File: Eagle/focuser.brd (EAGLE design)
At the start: 193 x 147.3 mm, 72 parts, among them IC1 L293D, IC2 L293D, IC4 L293D, IC5 7809, IC6 ULN2003AN, J5 RJ11, K1 G5L, K2 G5L, K3 G5L, K4 G5L, K5 G5L, Q1 IRFN44Z, Q2 IRFN44Z, Q3 IRFN44Z, Q4 IRFN44Z, U1 ARDUINO-MEGAFULL, X1 STEPPER1, X2 STEPPER2, X3 TOBU3, X4 TOBU3, X5 TOBU3, X6 TOBU3

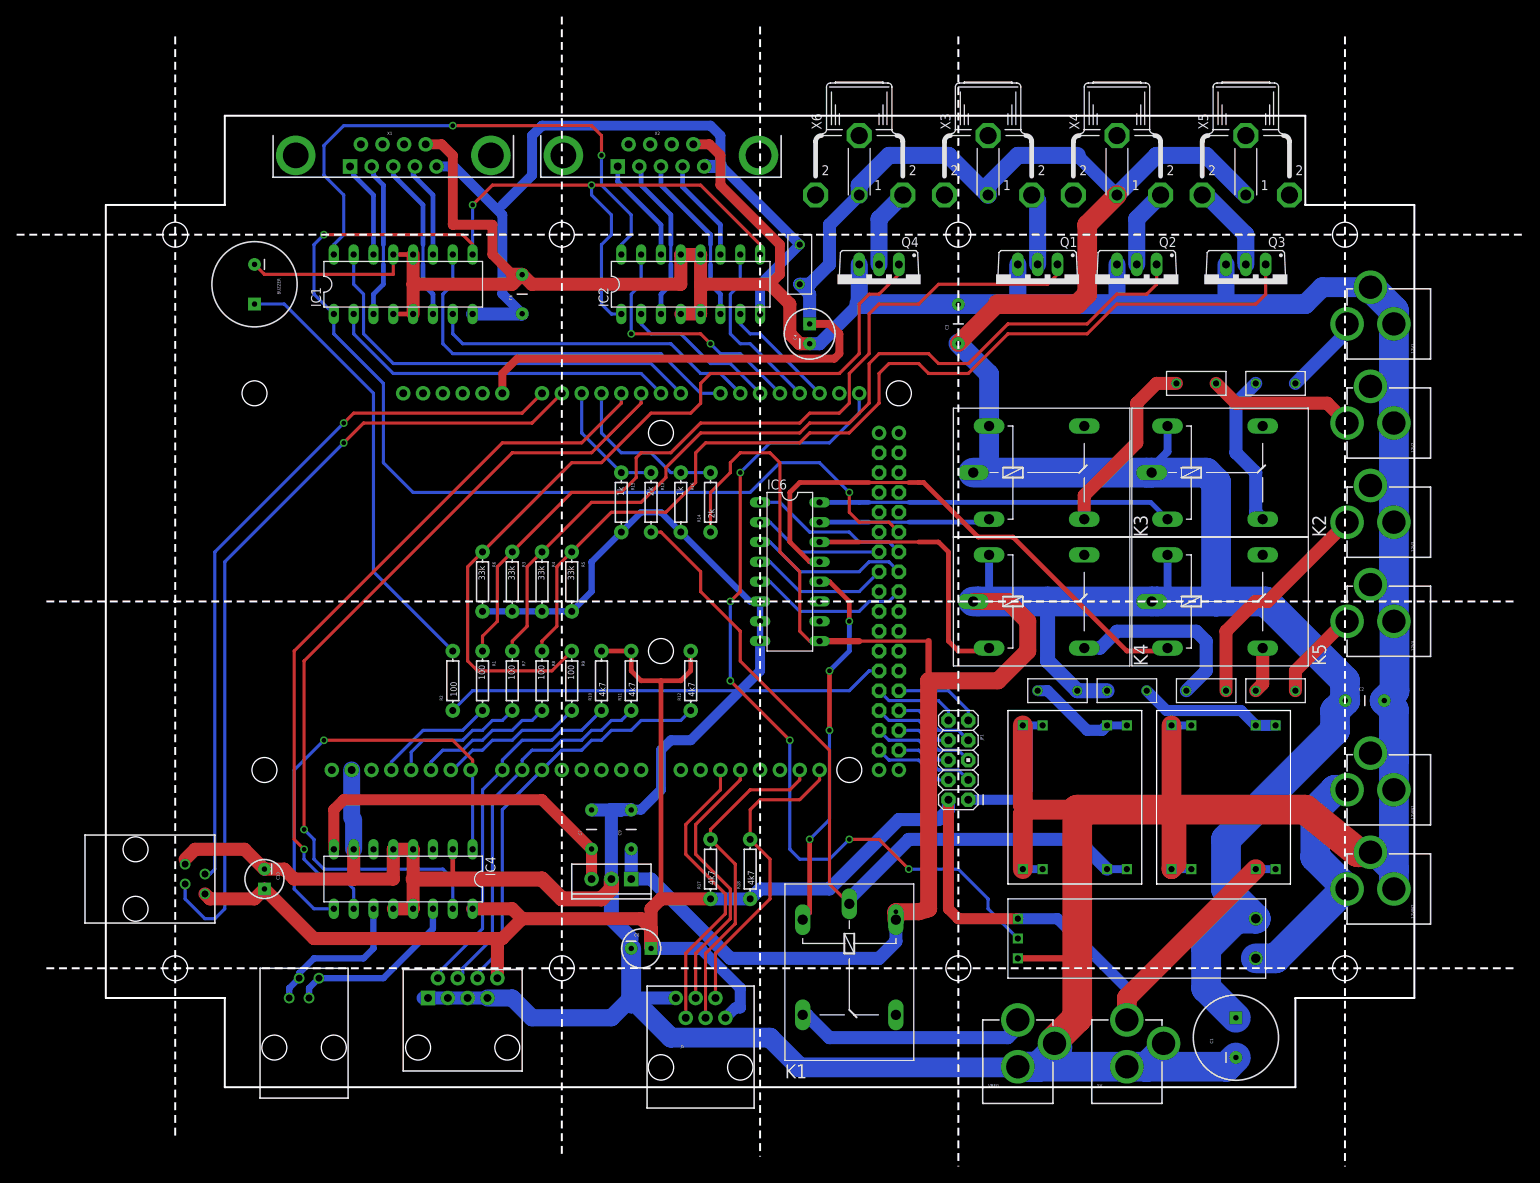
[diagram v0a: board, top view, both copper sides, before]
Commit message: PCB fixes
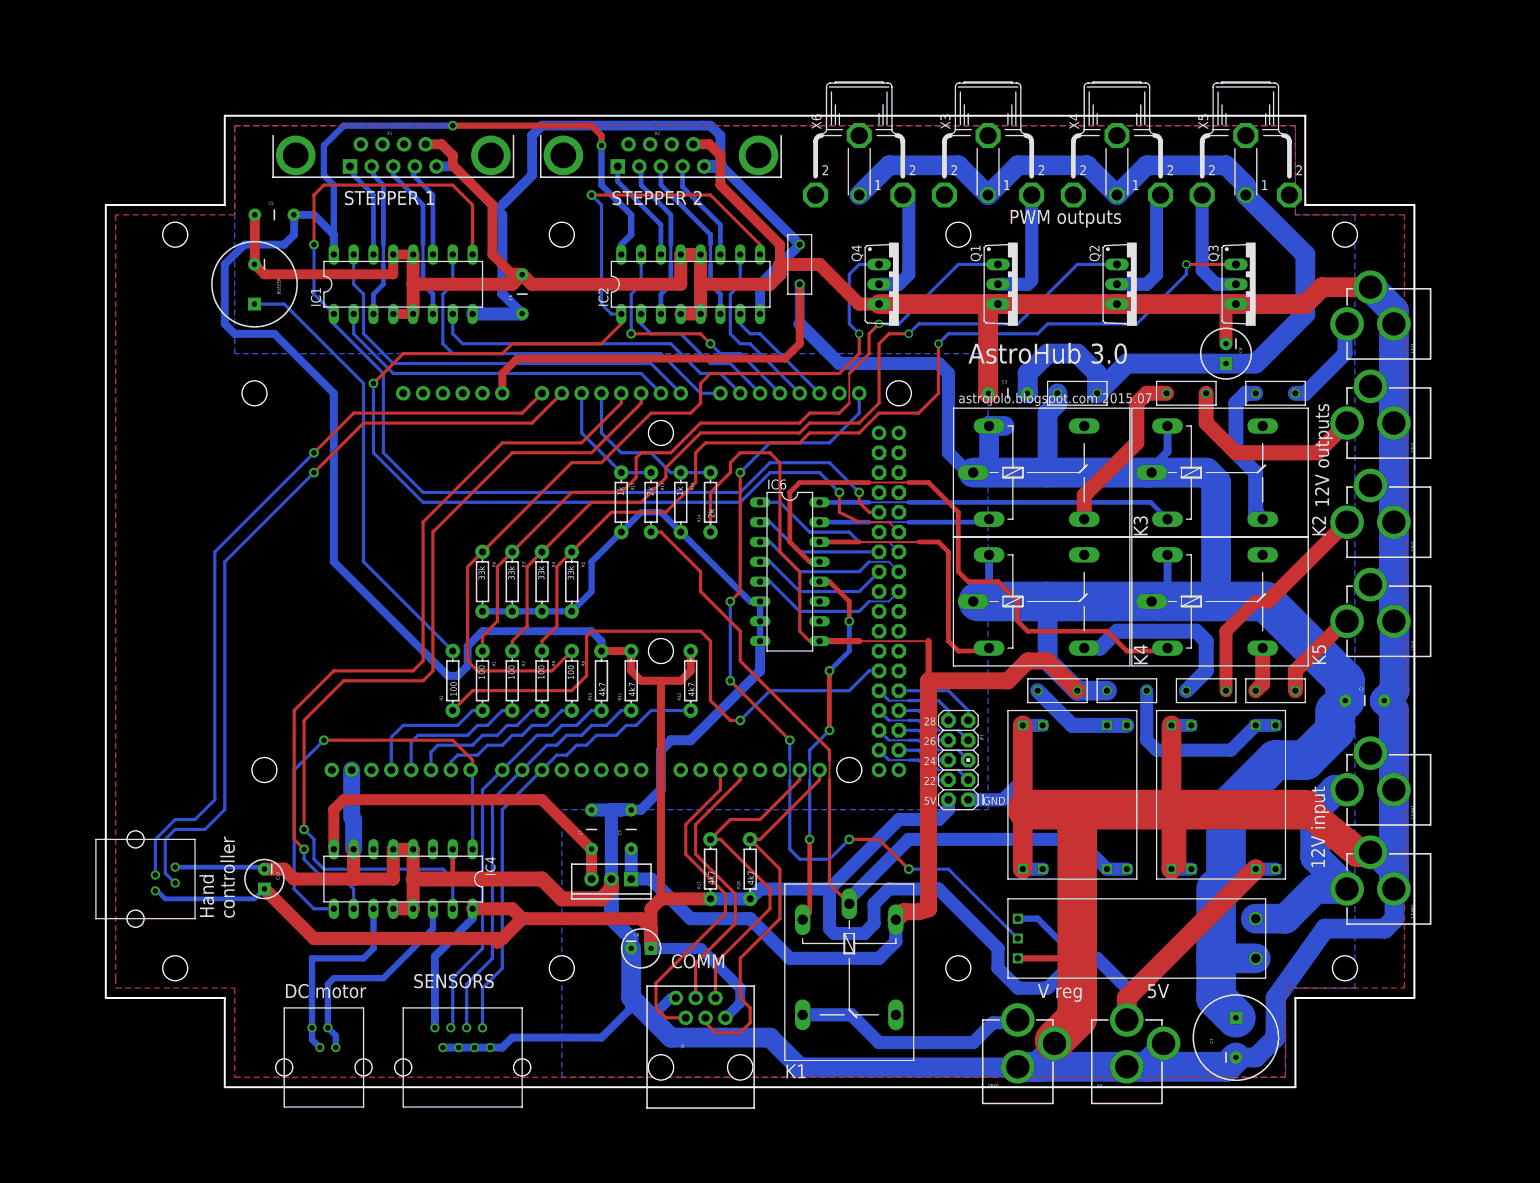
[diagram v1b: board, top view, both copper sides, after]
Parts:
- removed JP2: RJ45, SparkFun-Connectors:RJ45-8
- removed U$6: SW motor, SparkFun:RJ9
- removed U$7: Hand control, SparkFun:RJ9
- added C5: 100n, SparkFun:CAP-PTH-5MM
- added F8: 6A, SparkFun:PTC
- added U$4, U$5: RJ9, jolo-lib:RJ9
- added U$8: RJ45, jolo-lib:RJ45
- F1, F2, F3: value PTCPTH -> 2A
- F4, F5, F6, F7: value PTCPTH -> 4A
- J5: value RJ11 -> COMM
- JP1: value (none) -> EXT
- X3: value TOBU3 -> PWM1
- X4: value TOBU3 -> PWM2
- X5: value TOBU3 -> PWM3
- X6: value TOBU3 -> PWM4
- moved C4 53.4 mm to (142.2, 94.0), turned to 270 degrees
- moved C3 10.9 mm to (114.3, 88.9), turned to 0 degrees
- moved Q1 2.54 mm to (115.6, 102.9), turned to 270 degrees
- moved Q4 2.54 mm to (100.3, 102.9), turned to 270 degrees
- moved F5 1.80 mm to (137.2, 88.9)
- moved Q3 1.27 mm to (146.1, 102.9), turned to 270 degrees
- moved F4 1.27 mm to (148.6, 88.9)
- turned Q2 to 270 degrees
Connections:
- new net N$75: IC1.1, IC1.9, U1.46
- new net N$76: C3.2, C4.1, F8.P$2, X3.1, X4.1, X5.1, X6.1
- net +12V: now also F8.P$1, U$3.Z1; no longer C3.1, C4.1, U$3.Z2, X3.1, X4.1, X5.1, X6.1
- net +5V: now also C5.2, U$5.4, U$8.1; no longer JP2.8, U$7.4
- net GND: now also C3.1, C5.1, U$5.1, U$8.2, U$8.4, U$8.6, U$8.8; no longer C3.2, JP2.1, JP2.3, JP2.5, JP2.7, U$7.1
- net N$1: now also R18.P$2, U1.21; no longer R17.P$2, U1.20
- net N$12: no longer IC1.1, IC1.9
- net N$2: now also R17.P$2, U1.20; no longer R18.P$2, U1.21
- net N$26: now also U$3.Z2; no longer U$3.Z1
- net N$34: now also U$5.2; no longer U$7.2
- net N$44: now also U$5.3; no longer U$7.3
- net N$45: now also U$4.3, U$4.4; no longer U$6.3, U$6.4
- net N$51: now also U$4.1, U$4.2; no longer U$6.1, U$6.2
- net N$59: now also U$8.7; no longer JP2.6
- net N$65: now also U$8.5; no longer JP2.4
- net N$71: now also U$8.3; no longer JP2.2
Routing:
- net +5V: track 334.5 -> 492.8 mm
- net N$75: track 0.00 -> 135.5 mm, vias 0 -> 2
- net N$76: track 0.00 -> 125.2 mm
- net +12V: track 552.5 -> 467.3 mm, vias 1 -> 0
- net GND: track 833.5 -> 868.0 mm
- net N$12: track 197.2 -> 164.1 mm, vias 4 -> 3
- net N$46: track 56.7 -> 73.6 mm, vias 0 -> 1
- net N$42: track 106.8 -> 97.0 mm, vias 0 -> 1
- net N$69: track 18.4 -> 24.7 mm
- net N$35: track 9.21 -> 15.5 mm
- net N$52: track 18.9 -> 25.0 mm
- net N$41: track 114.5 -> 108.4 mm, vias 0 -> 1
- net N$59: track 52.3 -> 58.4 mm
- net N$1: track 42.4 -> 48.4 mm
- net N$31: track 94.0 -> 99.9 mm
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- added copper zone on layer 16, net +12V
- added copper zone on layer 1, net GND
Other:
- board size 193 x 147.3 mm -> 167.6 x 124.5 mm
- board text added: "12V input"
- board text added: "12V outputs"
- board text added: "22"
- board text added: "24"
- board text added: "26"
- board text added: "28"
- board text added: "5V"
- board text added: "AstroHub 3.0"
- board text added: "COMM"
- board text added: "DC motor"
- board text added: "GND"
- board text added: "Hand controller"
- board text added: "PWM outputs"
- board text added: "SENSORS"
- board text added: "STEPPER 1"
- board text added: "STEPPER 2"
- board text added: "V reg"
- board text added: "astrojolo.blogspot.com 2015.07"
